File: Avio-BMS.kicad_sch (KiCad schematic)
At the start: 6 parts

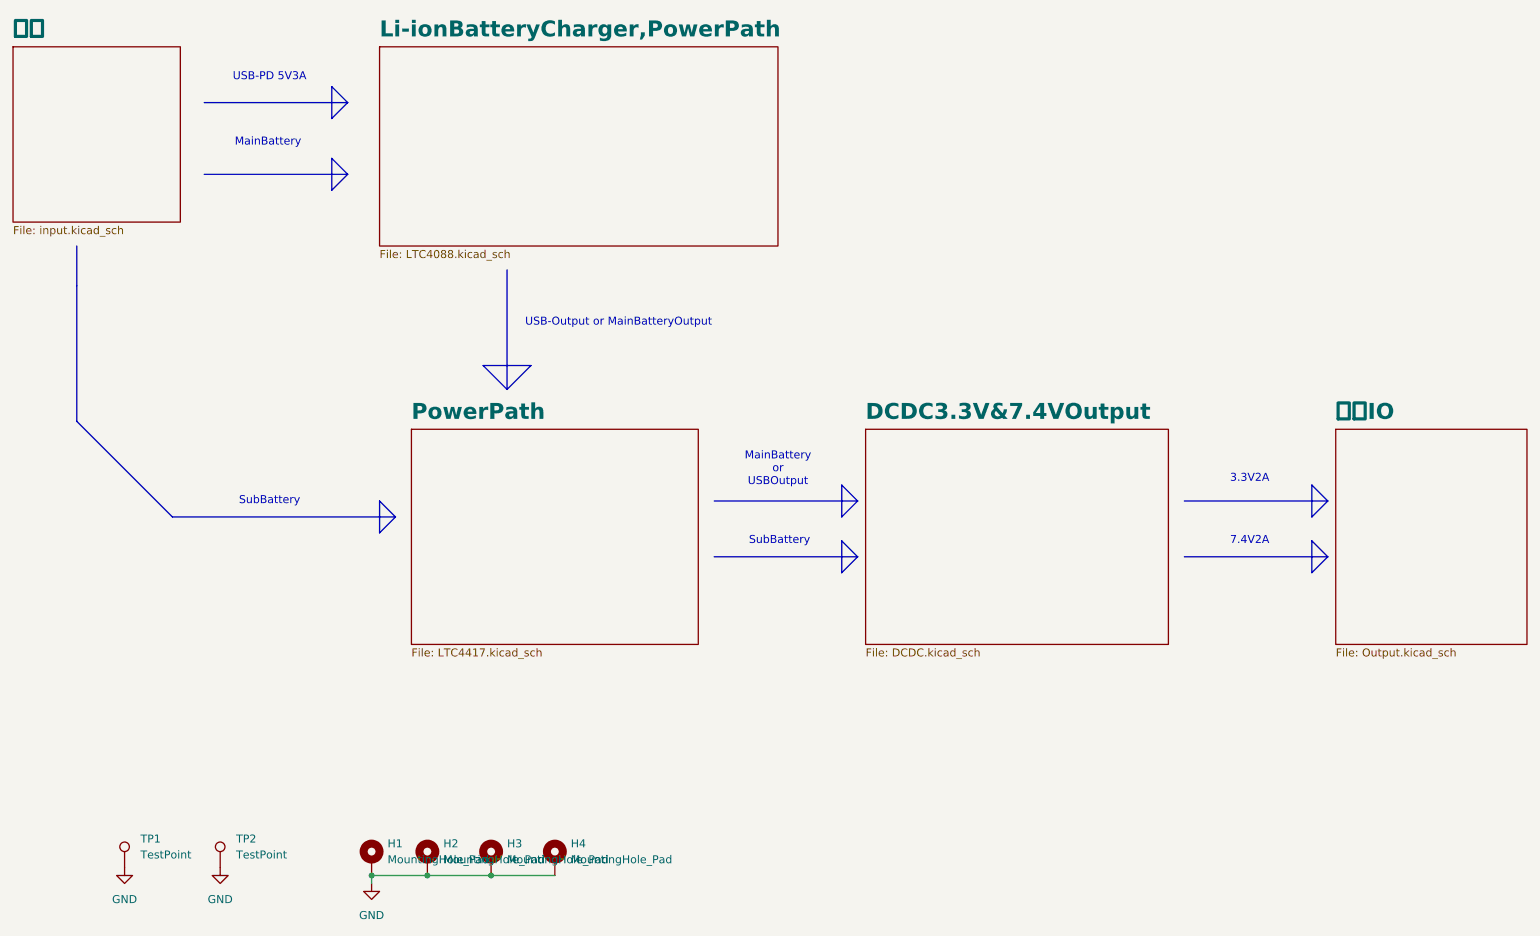
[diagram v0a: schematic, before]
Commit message: update sch
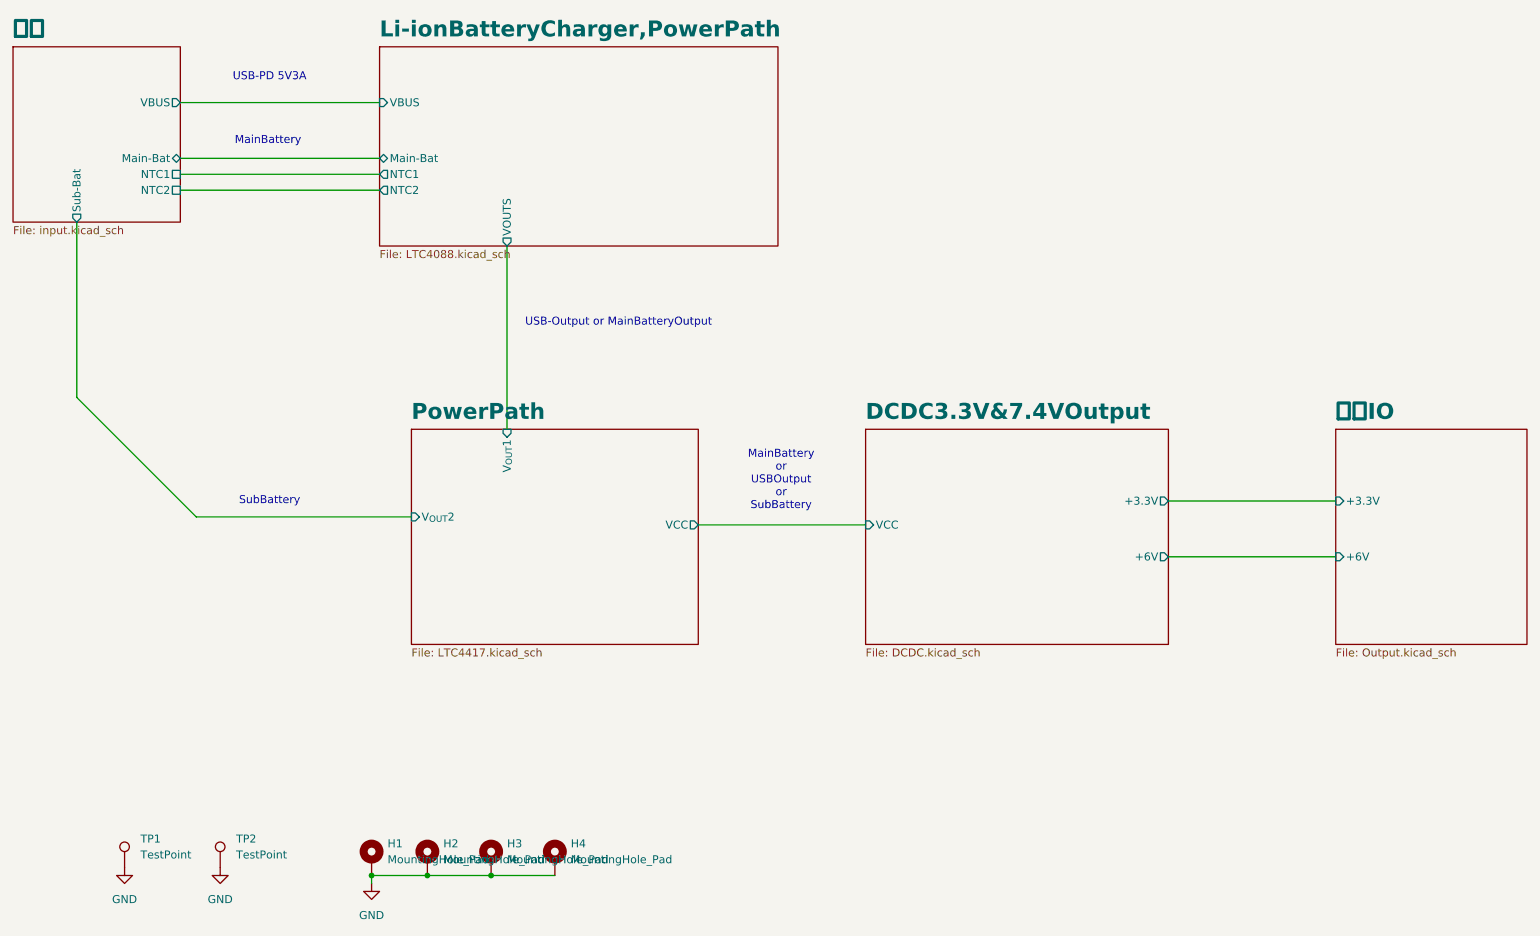
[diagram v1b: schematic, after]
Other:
- sheet DCDC3.3V&7.4VOutput ports: added +3.3V, +6V, VCC; removed none
- sheet Li-ionBatteryCharger,PowerPath ports: added Main-Bat, NTC1, NTC2, VBUS, VOUTS; removed none
- sheet PowerPath ports: added VCC, V_{OUT}1, V_{OUT}2; removed none
- sheet 入力 ports: added Main-Bat, NTC1, NTC2, Sub-Bat, VBUS; removed none
- sheet 出力IO ports: added +3.3V, +6V; removed none
- note added: "MainBattery or USBOutput or SubBattery"
- note removed: "3.3V2A"
- note removed: "7.4V2A"
- note removed: "MainBattery or USBOutput"
